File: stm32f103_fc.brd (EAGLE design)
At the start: 53 x 78.7 mm, 47 parts, among them IC1 STM32F10XCXT6, IC2 LD1117AS33TR, U2 9DoF IMU, Y1 8MHz, Y2 32.768MHz

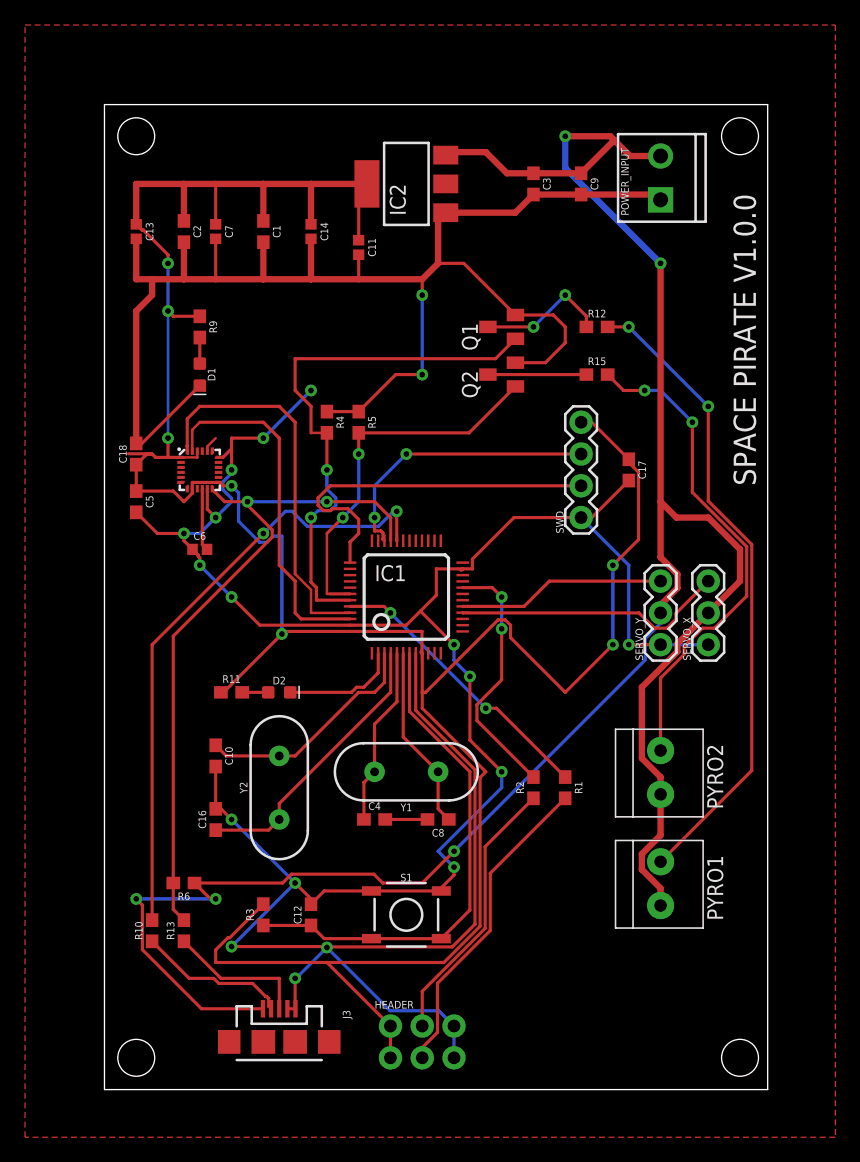
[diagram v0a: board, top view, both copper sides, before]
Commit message: done
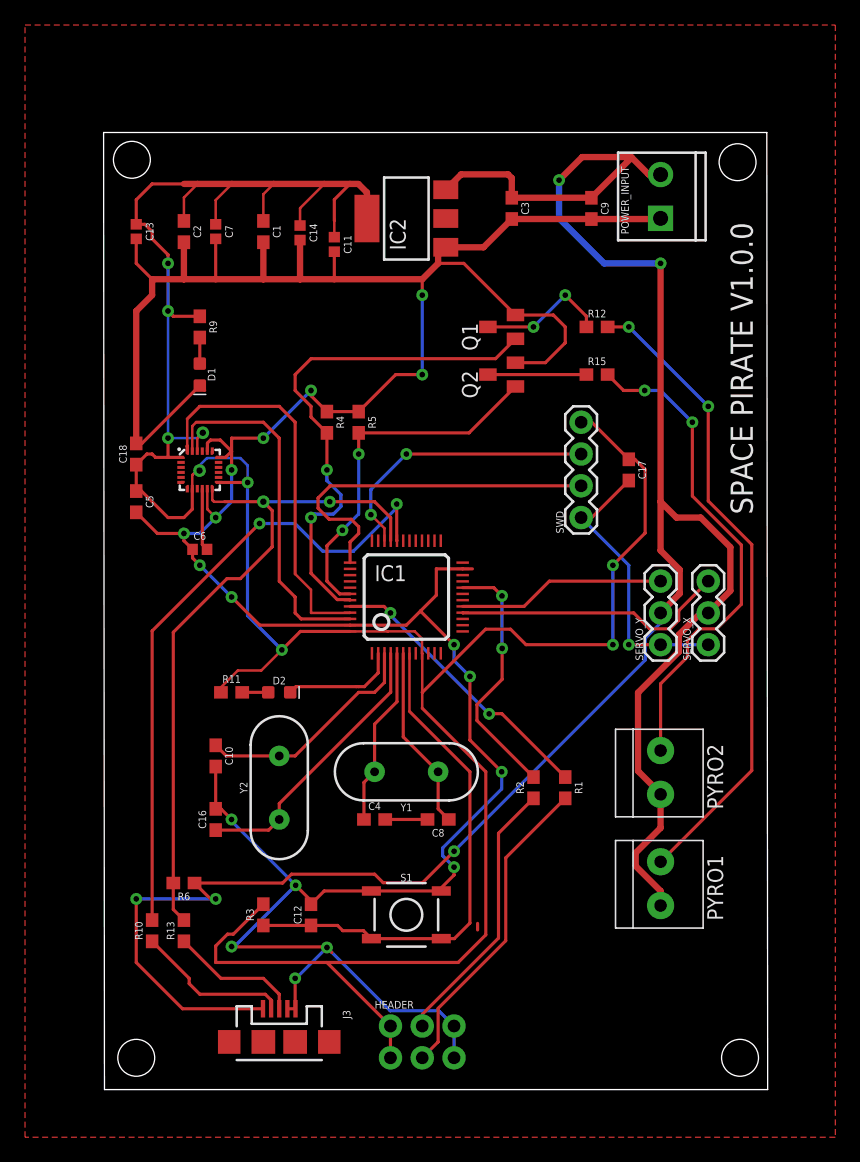
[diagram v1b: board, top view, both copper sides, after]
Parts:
- moved IC2 2.77 mm to (43.2, 81.1)
- moved C3 2.61 mm to (51.6, 81.9)
- moved C9 2.12 mm to (58.0, 81.9)
- moved C11 1.96 mm to (37.4, 79.0)
- moved POWER_INPUT 1.48 mm to (63.5, 81.1)
- moved C14 0.88 mm to (34.7, 79.9)
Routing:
- net GND: track 339.4 -> 293.0 mm
- net VCC3V3: track 221.3 -> 232.1 mm, vias 7 -> 9
- net 5V: track 180.3 -> 184.9 mm
- net PA11: track 49.3 -> 51.8 mm
- net PB7: track 43.9 -> 42.1 mm
- net N$8: track 11.3 -> 10.5 mm
- net PA12: track 54.9 -> 55.5 mm
- net RESET: track 40.4 -> 41.0 mm
- net PB6: track 29.8 -> 29.2 mm
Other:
- board size 53 x 78.7 mm -> 53.1 x 76.5 mm

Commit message: done final cam
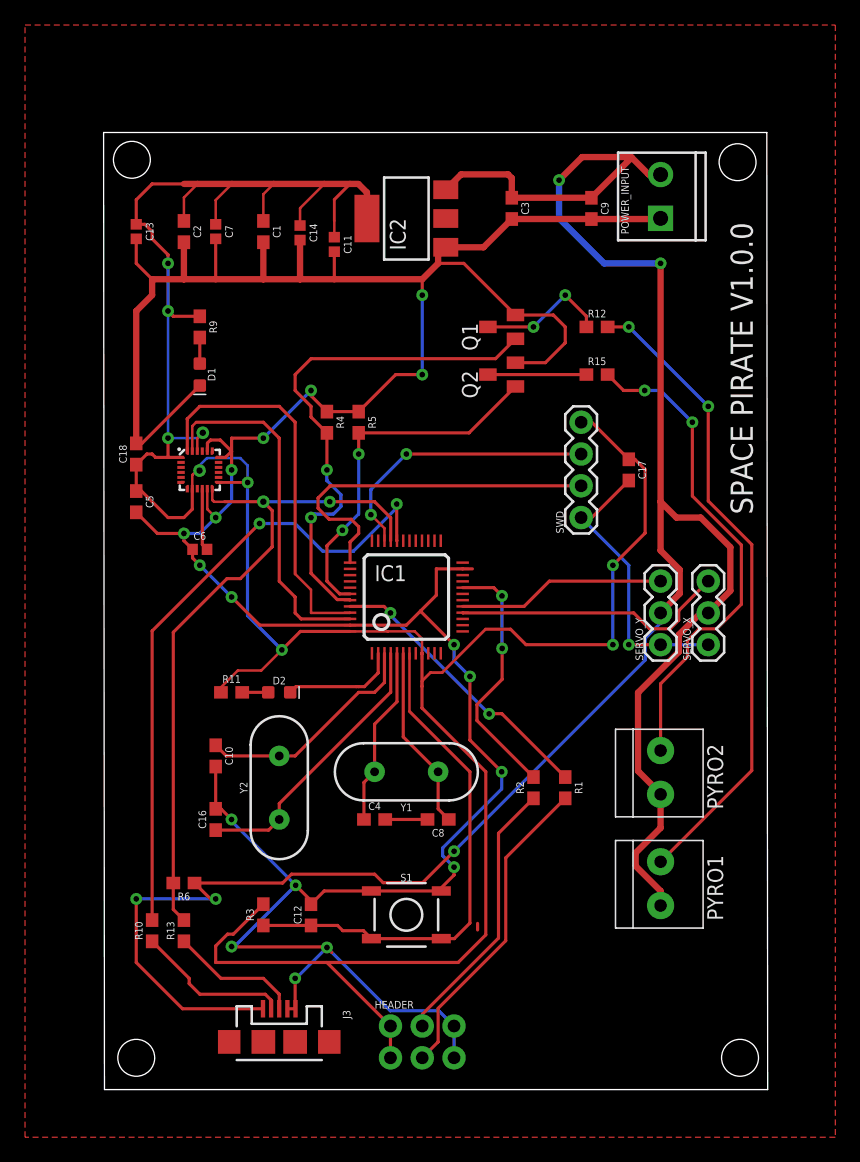
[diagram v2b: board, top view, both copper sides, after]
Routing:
- net VCC3V3: track 232.1 -> 231.0 mm
- net GND: track 293.0 -> 292.5 mm
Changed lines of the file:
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@@
 <wire x1="29.235909375" y1="83.82" x2="26.4898625" y2="83.82" width="0.508" layer="1"/>
 <wire x1="26.4898625" y1="83.82" x2="25.4" y2="83.82" width="0.508" layer="1"/>
-<wire x1="44.45" y1="41.91" x2="49.53" y2="36.83" width="0.254" layer="1"/>
 <wire x1="49.53" y1="36.83" x2="49.53" y2="23.799221875" width="0.254" layer="1"/>
 <wire x1="49.53" y1="23.799221875" x2="47.320778125" y2="21.59" width="0.254" layer="1"/>
@@
 <via x="59.69" y="46.99" extent="1-16" drill="0.45"/>
 <wire x1="51.5076" y1="48.228790625" x2="49.5118875" y2="48.228790625" width="0.254" layer="1"/>
-<wire x1="44.45" y1="43.18" x2="44.463096875" y2="43.18" width="0.254" layer="1"/>
-<wire x1="44.463096875" y1="43.18" x2="49.5118875" y2="48.228790625" width="0.254" layer="1"/>
 <wire x1="59.69" y1="46.99" x2="59.69" y2="53.34" width="0.254" layer="16"/>
 <via x="59.69" y="53.34" extent="1-16" drill="0.45"/>
@@
 <wire x1="62.26586875" y1="55.91586875" x2="62.26586875" y2="60.986296875" width="0.254" layer="1"/>
 <wire x1="59.69" y1="53.34" x2="62.26586875" y2="55.91586875" width="0.254" layer="1"/>
-<wire x1="28.2225" y1="59.96" x2="28.226746875" y2="59.955753125" width="0.254" layer="1"/>
-<wire x1="28.226746875" y1="59.955753125" x2="30.496009375" y2="59.955753125" width="0.254" layer="1"/>
 <via x="30.496009375" y="59.955753125" extent="1-16" drill="0.45"/>
 <via x="33.23" y="46.5724" extent="1-16" drill="0.45"/>
 <wire x1="30.496009375" y1="59.955753125" x2="30.4828625" y2="59.94260625" width="0.254" layer="16"/>
 <wire x1="34.7076" y1="48.05" x2="33.23" y2="46.5724" width="0.254" layer="1"/>
-<wire x1="40.03" y1="81.0538625" x2="39.37" y2="80.3938625" width="0.254" layer="1"/>
 <via x="24.13" y="77.47" extent="1-16" drill="0.45"/>
 <wire x1="24.13" y1="77.47" x2="24.13" y2="78.16013125" width="0.254" layer="1"/>
@@
 <wire x1="59.69" y1="46.99" x2="52.746390625" y2="46.99" width="0.254" layer="1"/>
 <wire x1="52.746390625" y1="46.99" x2="51.5076" y2="48.228790625" width="0.254" layer="1"/>
-<wire x1="44.43" y1="43.2" x2="44.45" y2="43.18" width="0.2032" layer="1"/>
 <wire x1="38.68" y1="48.05" x2="41.692409375" y2="48.05" width="0.2032" layer="1"/>
 <wire x1="44.43" y1="46.3" x2="44.43" y2="47.47629375" width="0.2032" layer="1"/>
@@
 <wire x1="43.850553125" y1="48.055740625" x2="41.69815" y2="48.055740625" width="0.2032" layer="1"/>
 <wire x1="41.69815" y1="48.055740625" x2="41.692409375" y2="48.05" width="0.2032" layer="1"/>
-<wire x1="44.43" y1="41.93" x2="44.45" y2="41.91" width="0.2032" layer="1"/>
-<wire x1="44.45" y1="41.91" x2="44.45" y2="43.166903125" width="0.2032" layer="1"/>
-<wire x1="44.45" y1="43.166903125" x2="44.463096875" y2="43.18" width="0.2032" layer="1"/>
-<wire x1="44.45" y1="43.166903125" x2="44.45" y2="46.28" width="0.2032" layer="1"/>
 <wire x1="44.45" y1="46.28" x2="44.43" y2="46.3" width="0.2032" layer="1"/>
 <wire x1="25.4" y1="80.86" x2="25.4" y2="82.7301375" width="0.2032" layer="1"/>
@@
 <wire x1="34.683253125" y1="81.88143125" x2="36.621821875" y2="83.82" width="0.2032" layer="1"/>
 <wire x1="37.421675" y1="79.563440625" x2="37.421675" y2="80.8708375" width="0.2032" layer="1"/>
-<wire x1="37.421675" y1="80.8708375" x2="37.421675" y2="81.0538625" width="0.2032" layer="1"/>
 <wire x1="39.34419375" y1="83.82" x2="39.37" y2="83.79419375" width="0.2032" layer="1"/>
 <wire x1="38.68" y1="48.05" x2="34.7076" y2="48.05" width="0.254" layer="1"/>
@@
 <wire x1="29.70589375" y1="44.926615625" x2="28.36" y2="43.580721875" width="0.2032" layer="1"/>
 <wire x1="28.36" y1="43.580721875" x2="28.36" y2="43.18" width="0.2032" layer="1"/>
-<wire x1="37.421675" y1="80.8708375" x2="37.421675" y2="82.567471875" width="0.254" layer="1"/>
 <wire x1="37.421675" y1="82.567471875" x2="38.674203125" y2="83.82" width="0.254" layer="1"/>
 <wire x1="39.37" y1="83.79419375" x2="40.03" y2="83.13419375" width="0.508" layer="1"/>
 <wire x1="40.03" y1="83.13419375" x2="40.03" y2="81.0538625" width="0.508" layer="1"/>
+<wire x1="44.43" y1="46.3" x2="44.43" y2="46.28298125" width="0.254" layer="1"/>
+<wire x1="44.43" y1="46.28298125" x2="44.43" y2="46.2802625" width="0.254" layer="1"/>
+<wire x1="44.43" y1="46.2802625" x2="44.43" y2="43.657159375" width="0.254" layer="1"/>
+<wire x1="44.43" y1="43.657159375" x2="44.43" y2="41.93" width="0.254" layer="1"/>
+<wire x1="44.43" y1="41.93" x2="49.53" y2="36.83" width="0.254" layer="1"/>
+<wire x1="44.43" y1="46.28298125" x2="44.43298125" y2="46.28" width="0.254" layer="1"/>
+<wire x1="44.43298125" y1="46.28" x2="44.45" y2="46.28" width="0.254" layer="1"/>
+<wire x1="44.43" y1="46.2802625" x2="44.4302625" y2="46.28" width="0.254" layer="1"/>
+<wire x1="44.4302625" y1="46.28" x2="44.43298125" y2="46.28" width="0.254" layer="1"/>
+<wire x1="30.4917625" y1="59.96" x2="30.496009375" y2="59.955753125" width="0.254" layer="1"/>
+<wire x1="49.5118875" y1="48.228790625" x2="46.0432375" y2="44.760140625" width="0.2286" layer="1"/>
+<wire x1="46.0432375" y1="44.760140625" x2="45.106328125" y2="44.760140625" width="0.2286" layer="1"/>
+<wire x1="45.106328125" y1="44.760140625" x2="44.43" y2="44.0838125" width="0.2286" layer="1"/>
+<wire x1="44.43" y1="44.0838125" x2="44.43" y2="43.657159375" width="0.2286" layer="1"/>
+<wire x1="28.2225" y1="59.96" x2="30.4917625" y2="59.96" width="0.2286" layer="1"/>
+<wire x1="37.421675" y1="80.8708375" x2="37.421675" y2="82.567471875" width="0.2286" layer="1"/>
 </signal>
 <signal name="N$1">
@@
 <wire x1="47.68" y1="53.05" x2="45.575" y2="53.05" width="0.254" layer="1"/>
 <wire x1="45.575" y1="53.05" x2="45.575" y2="50.945" width="0.254" layer="1"/>
-<wire x1="26.67" y1="67.703" x2="27.063" y2="67.31" width="0.254" layer="1"/>
 <wire x1="27.94" y1="79.43" x2="27.94" y2="76.2" width="0.254" layer="1"/>
 <wire x1="37.421675" y1="78.403440625" x2="37.421675" y2="76.2" width="0.254" layer="1"/>
@@
 <contactref element="SERVO_X" pad="2"/>
 <contactref element="SERVO_Y" pad="2"/>
-<wire x1="63.43" y1="84.636196875" x2="63.5" y2="84.566196875" width="0.508" layer="1"/>
 <wire x1="63.5" y1="84.566196875" x2="62.553803125" y2="84.566196875" width="0.508" layer="1"/>
 <wire x1="61.189803125" y1="85.930196875" x2="57.970659375" y2="82.711053125" width="0.508" layer="1"/>
@@
 <contactref element="IC1" pad="45"/>
 <contactref element="U2" pad="24"/>
-<wire x1="25.67" y1="62.88013125" x2="25.6656" y2="62.87573125" width="0.254" layer="1"/>
-<wire x1="25.6656" y1="62.81400625" x2="25.6656" y2="62.87573125" width="0.254" layer="1"/>
-<wire x1="25.67" y1="62.5125" x2="25.67" y2="62.88013125" width="0.254" layer="1"/>
-<wire x1="25.6656" y1="62.87573125" x2="25.6656" y2="65.0356" width="0.2032" layer="1"/>
 <wire x1="25.6656" y1="65.0356" x2="26.67" y2="66.04" width="0.254" layer="1"/>
 <wire x1="26.67" y1="66.04" x2="33.02" y2="66.04" width="0.254" layer="1"/>
@@
 <wire x1="35.56" y1="49.53" x2="35.56" y2="51.3747375" width="0.2032" layer="1"/>
 <wire x1="35.56" y1="51.3747375" x2="34.29" y2="52.6447375" width="0.2032" layer="1"/>
+<wire x1="25.67" y1="62.5125" x2="25.67" y2="65.0312" width="0.254" layer="1"/>
+<wire x1="25.67" y1="65.0312" x2="25.6656" y2="65.0356" width="0.254" layer="1"/>
 </signal>
 <signal name="PB9">
